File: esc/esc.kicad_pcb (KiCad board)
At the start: 2 copper layers, 90 x 90 mm, 45 parts, among them J1 Conn_01x04, J2 Conn_01x04, J3 Conn_01x04, J4 Conn_01x01, J5 Conn_01x01, J6 Conn_01x03, J7 Conn_01x02, J8 Conn_01x02, J9 Conn_01x02, Q1 FDS2734, Q2 FDS2734, Q3 FDS2734, Q4 FDS2734, Q5 FDS2734, Q6 FDS2734, U1 STM32F051C8Tx, U2 KA78M05_TO252, U3 REGULAR-7133-1, U4 IR2103, U5 IR2103, U6 IR2103

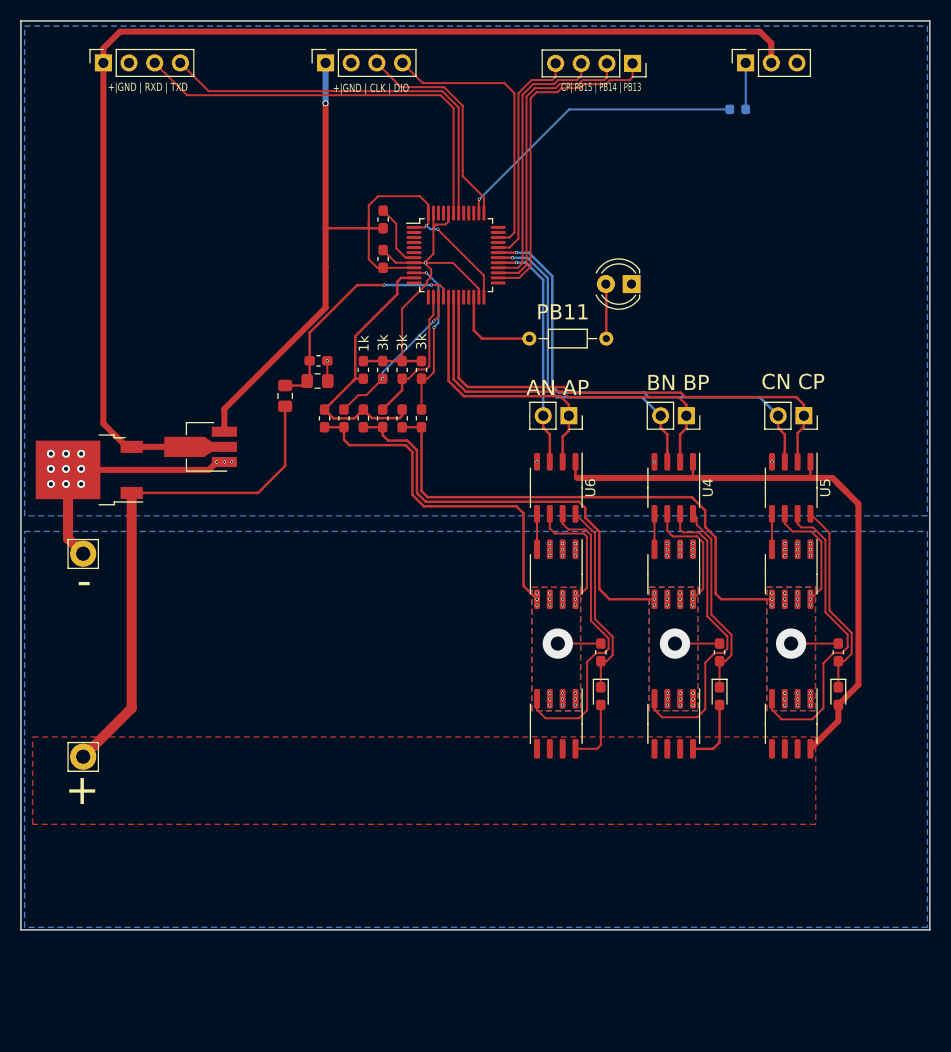
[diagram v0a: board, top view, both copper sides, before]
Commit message: 19号已经打样
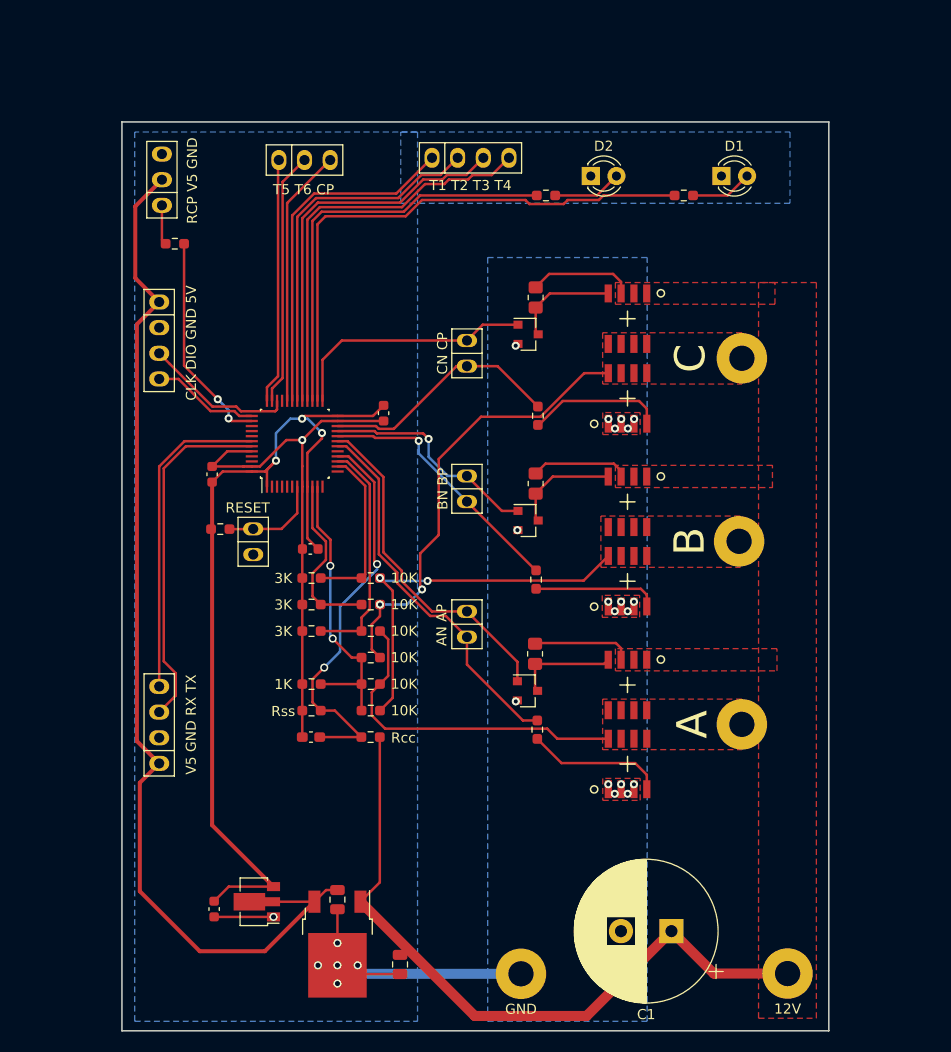
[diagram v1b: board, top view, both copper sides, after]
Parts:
- removed D3, D4: D, Diode_SMD:D_0603_1608Metric_Pad1.05x0.95mm_HandSolder
- removed U4, U5, U6: IR2103, Package_SO:SO-8_3.9x4.9mm_P1.27mm
- added C7: C, Capacitor_SMD:C_0805_2012Metric, F.Cu at (57.5, 113.4)
- added C8: C, Capacitor_SMD:C_0805_2012Metric, F.Cu at (51.3, 107.0)
- added J10: RCP V5 GND, footprint:CONN3-P2.54-DR1.0-W1.5, F.Cu at (34.0, 35.7)
- added J11: AN AP, footprint:CONN2-P2.54-DR1.0-W1.3, F.Cu at (64.2, 79.7)
- added J12: BN BP, footprint:CONN2-P2.54-DR1.0-W1.3, F.Cu at (64.2, 66.3)
- added J13: CN CP, footprint:CONN2-P2.54-DR1.0-W1.3, F.Cu at (64.2, 52.9)
- added J14: CLK DIO GND 5V, footprint:CONN4-P2.54-DR1.0-W1.5, F.Cu at (33.7, 51.6)
- added Q7: 2N3055, Package_TO_SOT_SMD:SOT-23, F.Cu at (70.2, 51.0)
- added Q8: nfet, footprint:SOIC-8, F.Cu at (80.1, 57.4)
- added Q9: pfet, footprint:SOIC-8, F.Cu at (80.1, 49.5)
- added R15: 1K, Resistor_SMD:R_0603_1608Metric_Pad0.98x0.95mm_HandSolder, F.Cu at (72.0, 37.3)
- added R16: 1K, Resistor_SMD:R_0603_1608Metric_Pad0.98x0.95mm_HandSolder, F.Cu at (35.2, 42.1)
- added R17: R, Resistor_SMD:R_0603_1608Metric_Pad0.98x0.95mm_HandSolder, F.Cu at (71.1, 90.2)
- added R18: 1K, Resistor_SMD:R_0805_2012Metric_Pad1.20x1.40mm_HandSolder, F.Cu at (70.9, 82.7)
- added R19: R, Resistor_SMD:R_0603_1608Metric_Pad0.98x0.95mm_HandSolder, F.Cu at (71.0, 75.3)
- added R20: 1K, Resistor_SMD:R_0805_2012Metric_Pad1.20x1.40mm_HandSolder, F.Cu at (71.0, 65.8)
- added R21: R, Resistor_SMD:R_0603_1608Metric_Pad0.98x0.95mm_HandSolder, F.Cu at (71.2, 59.1)
- added R22: 1K, Resistor_SMD:R_0805_2012Metric_Pad1.20x1.40mm_HandSolder, F.Cu at (71.0, 47.4)
- C1: footprint Capacitor_SMD:C_0603_1608Metric_Pad1.05x0.95mm_HandSolder -> Capacitor_THT:CP_Radial_D14.0mm_P5.00mm
- C2: footprint Capacitor_SMD:C_0603_1608Metric -> Capacitor_SMD:C_0603_1608Metric_Pad1.08x0.95mm_HandSolder; moved to F.Cu
- C3, C4, C5, C6: footprint Capacitor_SMD:C_0603_1608Metric_Pad1.05x0.95mm_HandSolder -> Capacitor_SMD:C_0603_1608Metric
- D1: footprint LED_THT:LED_D4.0mm -> LED_THT:LED_D3.0mm
- D2: value D -> LED; footprint Diode_SMD:D_0603_1608Metric_Pad1.05x0.95mm_HandSolder -> LED_THT:LED_D3.0mm
- J1: value Conn_01x04 -> 12V; footprint Connector_PinSocket_2.54mm:PinSocket_1x04_P2.54mm_Vertical -> MountingHole:MountingHole_2.5mm_Pad
- J2: value Conn_01x04 -> GND; footprint Connector_PinSocket_2.54mm:PinSocket_1x04_P2.54mm_Vertical -> MountingHole:MountingHole_2.5mm_Pad
- J3: value Conn_01x04 -> A; footprint Connector_PinSocket_2.54mm:PinSocket_1x04_P2.54mm_Vertical -> MountingHole:MountingHole_2.5mm_Pad
- J4: value Conn_01x01 -> B; footprint Connector_Pin:Pin_D1.4mm_L8.5mm_W2.8mm_FlatFork -> MountingHole:MountingHole_2.5mm_Pad
- J5: value Conn_01x01 -> C; footprint Connector_Pin:Pin_D1.4mm_L8.5mm_W2.8mm_FlatFork -> MountingHole:MountingHole_2.5mm_Pad
- J6: value Conn_01x03 -> RESET; footprint Connector_PinSocket_2.54mm:PinSocket_1x03_P2.54mm_Vertical -> footprint:CONN2-P2.54-DR1.0-W1.3
- J7: value Conn_01x02 -> V5 GND RX TX; footprint Connector_PinSocket_2.54mm:PinSocket_1x02_P2.54mm_Vertical -> footprint:CONN4-P2.54-DR1.0-W1.5
- J8: value Conn_01x02 -> T1 T2 T3 T4; footprint Connector_PinSocket_2.54mm:PinSocket_1x02_P2.54mm_Vertical -> footprint:CONN4-P2.54-DR1.0-W1.5
- J9: value Conn_01x02 -> T5 T6 CP; footprint Connector_PinSocket_2.54mm:PinSocket_1x02_P2.54mm_Vertical -> footprint:CONN3-P2.54-DR1.0-W1.5
- Q1, Q4: value FDS2734 -> 2N3055; footprint Package_SO:SOIC-8_3.9x4.9mm_P1.27mm -> Package_TO_SOT_SMD:SOT-23
- Q2, Q5: value FDS2734 -> nfet; footprint Package_SO:SOIC-8_3.9x4.9mm_P1.27mm -> footprint:SOIC-8
- Q3, Q6: value FDS2734 -> pfet; footprint Package_SO:SOIC-8_3.9x4.9mm_P1.27mm -> footprint:SOIC-8
- R1: value 1k -> Rcc; footprint Resistor_SMD:R_0603_1608Metric_Pad1.05x0.95mm_HandSolder -> Resistor_SMD:R_0603_1608Metric_Pad0.98x0.95mm_HandSolder
- R10: value 3k -> 10K; footprint Resistor_SMD:R_0603_1608Metric_Pad1.05x0.95mm_HandSolder -> Resistor_SMD:R_0603_1608Metric_Pad0.98x0.95mm_HandSolder
- R11, R14: value 20k -> 1K; footprint Resistor_SMD:R_0603_1608Metric_Pad1.05x0.95mm_HandSolder -> Resistor_SMD:R_0603_1608Metric_Pad0.98x0.95mm_HandSolder
- R12: value 1k -> 1K; footprint Resistor_SMD:R_0603_1608Metric_Pad1.05x0.95mm_HandSolder -> Resistor_SMD:R_0603_1608Metric_Pad0.98x0.95mm_HandSolder
- R13, R5, R7, R9: value 20k -> 10K; footprint Resistor_SMD:R_0603_1608Metric_Pad1.05x0.95mm_HandSolder -> Resistor_SMD:R_0603_1608Metric_Pad0.98x0.95mm_HandSolder
- R2: value 1K -> Rss; footprint Resistor_THT:R_Axial_DIN0204_L3.6mm_D1.6mm_P7.62mm_Horizontal -> Resistor_SMD:R_0603_1608Metric_Pad0.98x0.95mm_HandSolder
- R3: value 2K -> 10K; footprint Resistor_SMD:R_0805_2012Metric_Pad1.15x1.40mm_HandSolder -> Resistor_SMD:R_0603_1608Metric_Pad0.98x0.95mm_HandSolder
- R4: value 2K -> 3K; footprint Resistor_SMD:R_0805_2012Metric_Pad1.15x1.40mm_HandSolder -> Resistor_SMD:R_0603_1608Metric_Pad0.98x0.95mm_HandSolder
- R6, R8: value 3k -> 3K; footprint Resistor_SMD:R_0603_1608Metric_Pad1.05x0.95mm_HandSolder -> Resistor_SMD:R_0603_1608Metric_Pad0.98x0.95mm_HandSolder
- U1: footprint Package_QFP:LQFP-48_7x7mm_P0.5mm -> footprint:QFP-48_P0.5mm_W0.22
- U2: value KA78M05_TO252 -> L7805
- U3: footprint Package_TO_SOT_SMD:SOT-89-3_Handsoldering -> Package_TO_SOT_SMD:SOT-89-3
- moved J2 92.3 mm to (69.5, 114.4), turned to 0 degrees
- moved J1 91.4 mm to (95.9, 114.3), turned to 0 degrees
- moved J3 91.0 mm to (91.4, 89.7), turned to 0 degrees
- moved C2 75.2 mm to (48.7, 90.9)
- moved C1 72.4 mm to (84.4, 110.1), turned to 180 degrees
- moved J4 68.4 mm to (91.1, 71.5)
- moved J5 68.0 mm to (91.4, 53.4)
- moved J6 68.0 mm to (43.0, 71.6), turned to 270 degrees
- moved C5 64.5 mm to (38.9, 64.9)
- moved J9 55.6 mm to (48.1, 33.8), turned to 0 degrees
- moved C3 55.3 mm to (39.1, 107.9), turned to 270 degrees
- moved D2 53.1 mm to (76.4, 35.4), turned to 0 degrees
- moved U2 53.0 mm to (51.3, 111.4), turned to 270 degrees
- moved R1 51.3 mm to (54.6, 90.9), turned to 0 degrees
- moved J7 50.8 mm to (33.7, 89.7), turned to 90 degrees
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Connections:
- C1 pad 1: +3V3 -> VCC
- C2 pad 1: Net-(C2-Pad1) -> V_SAMPLE
- C2 pad 2: RCP -> GND
- C3 pad 1: V_SAMPLE -> +3V3
- C4 pad 1: Net-(C4-Pad1) -> +3V3
- C4 pad 2: /BOUT -> GND
- C5 pad 1: Net-(C5-Pad1) -> +3V3
- C5 pad 2: /COUT -> GND
- C6 pad 1: Net-(C6-Pad1) -> +3V3
- C6 pad 2: /AOUT -> GND
- D2 pad 1: Net-(C4-Pad1) -> GND
- D2 pad 2: VCC -> Net-(D2-Pad2)
- J1 pad 1: /PB13 -> VCC
- J2 pad 1: +3V3 -> GND
- J3 pad 1: +5V -> OUT_A
- J4 pad 1: VCC -> OUT_B
- J5 pad 1: GND -> OUT_C
- J6 pad 1: Net-(C2-Pad1) -> RESET
- J6 pad 2: +5V -> GND
- J7 pad 1: AP -> +5V
- J7 pad 2: AN -> GND
- J8 pad 1: BP -> TEST1
- J8 pad 2: BN -> TEST2
- J9 pad 1: CP -> TEST5
- J9 pad 2: CN -> TEST6
- Q1 pad 1: /BOUT -> AP
- Q1 pad 2: /BOUT -> GND
- Q1 pad 3: /BOUT -> Net-(Q1-Pad3)
- Q2 pad 5: /BOUT -> OUT_A
- Q2 pad 6: /BOUT -> OUT_A
- Q2 pad 7: /BOUT -> OUT_A
- Q2 pad 8: /BOUT -> OUT_A
- Q3 pad 1: /COUT -> VCC
- Q3 pad 2: /COUT -> VCC
- Q3 pad 3: /COUT -> VCC
- Q3 pad 4: Net-(Q3-Pad4) -> Net-(Q1-Pad3)
- Q3 pad 5: VCC -> OUT_A
- Q3 pad 6: VCC -> OUT_A
- Q3 pad 7: VCC -> OUT_A
- Q3 pad 8: VCC -> OUT_A
- Q4 pad 1: GND -> BP
- Q4 pad 3: GND -> Net-(Q4-Pad3)
- Q5 pad 1: /AOUT -> GND
- Q5 pad 2: /AOUT -> GND
- Q5 pad 3: /AOUT -> GND
- Q5 pad 5: VCC -> OUT_B
- Q5 pad 6: VCC -> OUT_B
- Q5 pad 7: VCC -> OUT_B
- Q5 pad 8: VCC -> OUT_B
- Q6 pad 1: GND -> VCC
- Q6 pad 2: GND -> VCC
- Q6 pad 3: GND -> VCC
- Q6 pad 4: Net-(Q6-Pad4) -> Net-(Q4-Pad3)
- Q6 pad 5: /AOUT -> OUT_B
- Q6 pad 6: /AOUT -> OUT_B
- Q6 pad 7: /AOUT -> OUT_B
- Q6 pad 8: /AOUT -> OUT_B
- R1 pad 1: Net-(R1-Pad1) -> V_SAMPLE
- R1 pad 2: +3V3 -> VCC
- R10 pad 1: Fa -> Fabc
- R10 pad 2: GND -> OUT_B
- R11 pad 1: /AOUT -> GND
- R12 pad 1: Fabc -> RESET
- R12 pad 2: GND -> +3V3
- R13 pad 1: /BOUT -> Fabc
- R13 pad 2: Fabc -> OUT_C
- R14 pad 1: /COUT -> Net-(D1-Pad2)
- R14 pad 2: Fabc -> LED1
- R2 pad 1: Net-(D1-Pad2) -> GND
- R2 pad 2: /LED -> V_SAMPLE
- R3 pad 1: VCC -> Fa
- R3 pad 2: V_SAMPLE -> OUT_A
- R4 pad 1: V_SAMPLE -> GND
- R4 pad 2: GND -> Fa
- R5 pad 1: /COUT -> Fb
- R5 pad 2: Fc -> OUT_B
- R6 pad 1: Fc -> GND
- R6 pad 2: GND -> Fb
- R7 pad 1: /BOUT -> Fc
- R7 pad 2: Fb -> OUT_C
- R8 pad 1: Fb -> GND
- R8 pad 2: GND -> Fc
- R9 pad 1: /AOUT -> Fabc
- R9 pad 2: Fa -> OUT_A
- U1 pad 12: (no net) -> Net-(U1-Pad12)
- U1 pad 13: (no net) -> Net-(U1-Pad13)
- U1 pad 17: AP -> Net-(U1-Pad17)
- U1 pad 18: BP -> AN
- U1 pad 19: CP -> AP
- U1 pad 2: (no net) -> Net-(U1-Pad2)
- U1 pad 20: (no net) -> BN
- U1 pad 21: (no net) -> BP
- U1 pad 22: /LED -> CN
- U1 pad 25: (no net) -> CP
- U1 pad 26: /PB13 -> LED1
- U1 pad 27: /PB14 -> LED2
- U1 pad 28: /PB15 -> TEST4
- U1 pad 29: AN -> TEST3
- U1 pad 3: (no net) -> Net-(U1-Pad3)
- U1 pad 30: BN -> TEST2
- U1 pad 31: CN -> TEST1
- U1 pad 32: /CP-OUT -> CPOUT
- U1 pad 33: (no net) -> Net-(U1-Pad33)
- U1 pad 34: /SWDIO -> SWDIO
- U1 pad 35: (no net) -> TEST6
- U1 pad 36: (no net) -> TEST5
- U1 pad 37: /SWCLK -> SWCLK
- U1 pad 39: (no net) -> Net-(U1-Pad39)
- U1 pad 4: (no net) -> Net-(U1-Pad4)
- U1 pad 40: (no net) -> Net-(U1-Pad40)
- U1 pad 41: (no net) -> Net-(U1-Pad41)
- U1 pad 42: /TXD -> TXD
- U1 pad 43: /RXD -> RXD
- U1 pad 45: (no net) -> Net-(U1-Pad45)
- U1 pad 46: (no net) -> Net-(U1-Pad46)
- U1 pad 5: (no net) -> Net-(U1-Pad5)
- U1 pad 6: (no net) -> Net-(U1-Pad6)
- U1 pad 7: Net-(R1-Pad1) -> RESET
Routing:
- net /COUT: track 67.8 -> 0.00 mm, vias 22 -> 0
- net /BOUT: track 58.9 -> 0.00 mm, vias 22 -> 0
- net LED1: track 0.00 -> 54.4 mm
- net /AOUT: track 51.9 -> 0.00 mm, vias 22 -> 0
- net OUT_C: track 0.00 -> 44.8 mm, vias 0 -> 2
- net /RXD: track 41.8 -> 0.00 mm
- net LED2: track 0.00 -> 41.1 mm
- net TEST4: track 0.00 -> 40.4 mm
- net /TXD: track 39.8 -> 0.00 mm
- net TEST3: track 0.00 -> 38.5 mm
- net OUT_B: track 0.00 -> 37.9 mm, vias 0 -> 2
- net TEST2: track 0.00 -> 36.5 mm
- net RXD: track 0.00 -> 34.9 mm
- net TEST1: track 0.00 -> 34.6 mm
- net OUT_A: track 0.00 -> 33.7 mm
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- added copper zone on F.Cu, net GND
- added copper zone on F.Cu, net OUT_A
- added copper zone on F.Cu, net OUT_B
- added copper zone on F.Cu, net OUT_C
- removed copper zone on B.Cu, net /AOUT
- removed copper zone on F.Cu, net /AOUT
- removed copper zone on B.Cu, net /BOUT
- removed copper zone on F.Cu, net /BOUT
- removed copper zone on B.Cu, net /COUT
- removed copper zone on F.Cu, net /COUT
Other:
- board size 90 x 90 mm -> 70 x 90 mm
- net class power added: clearance 0.2, trace_width 0.4, via_dia 0.8, via_drill 0.4
- board text removed: "+"
- board text removed: "+|GND | CLK | DIO"
- board text removed: "+|GND | RXD | TXD"
- board text removed: "-"
- board text removed: "AN AP"
- board text removed: "BN BP"
- board text removed: "CN CP"
- board text removed: "CP| PB15 | PB14 | PB13"
- board text removed: "PB11"
